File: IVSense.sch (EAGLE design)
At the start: 18 parts

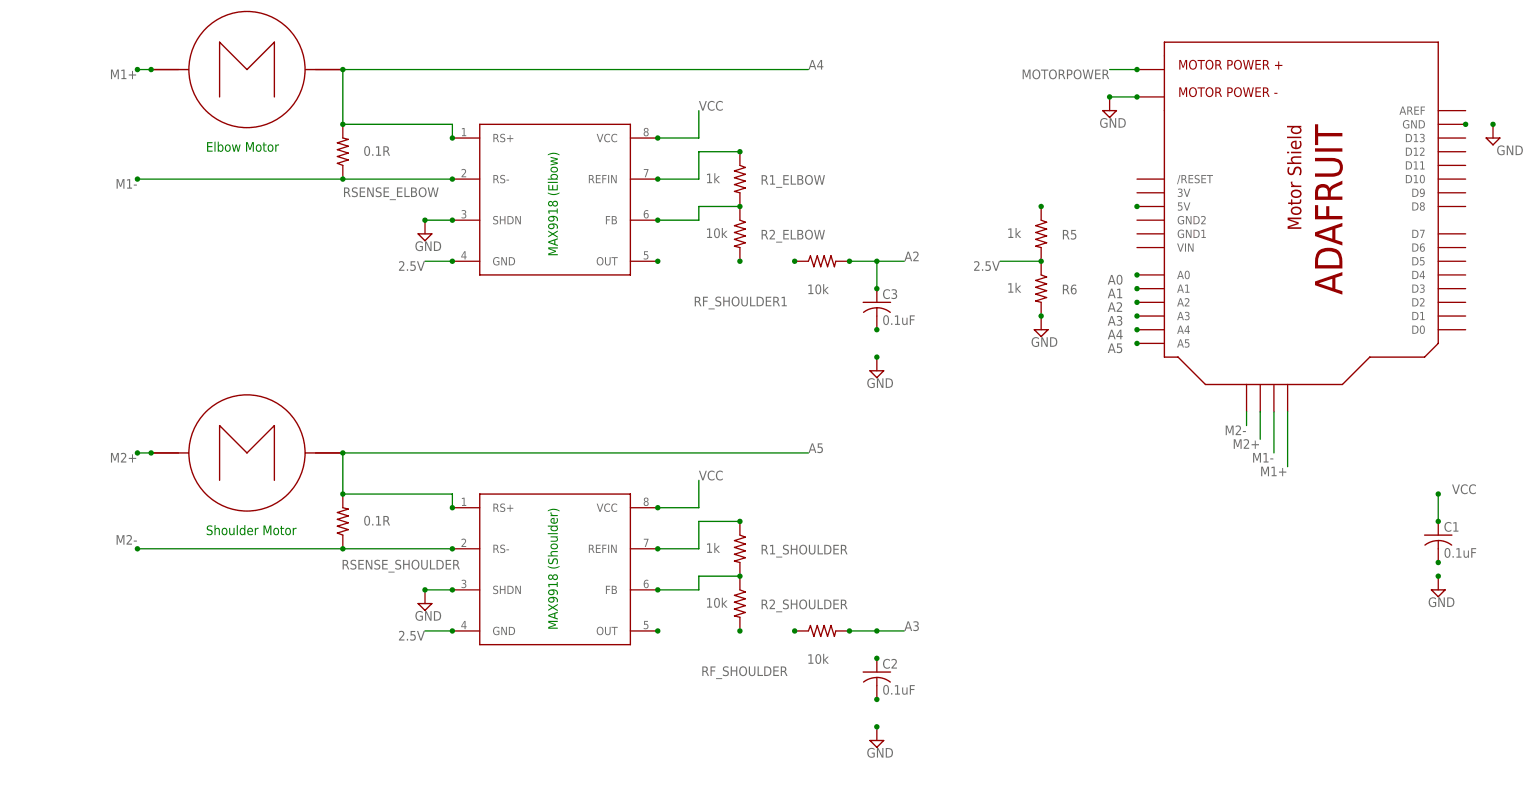
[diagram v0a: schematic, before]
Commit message: update
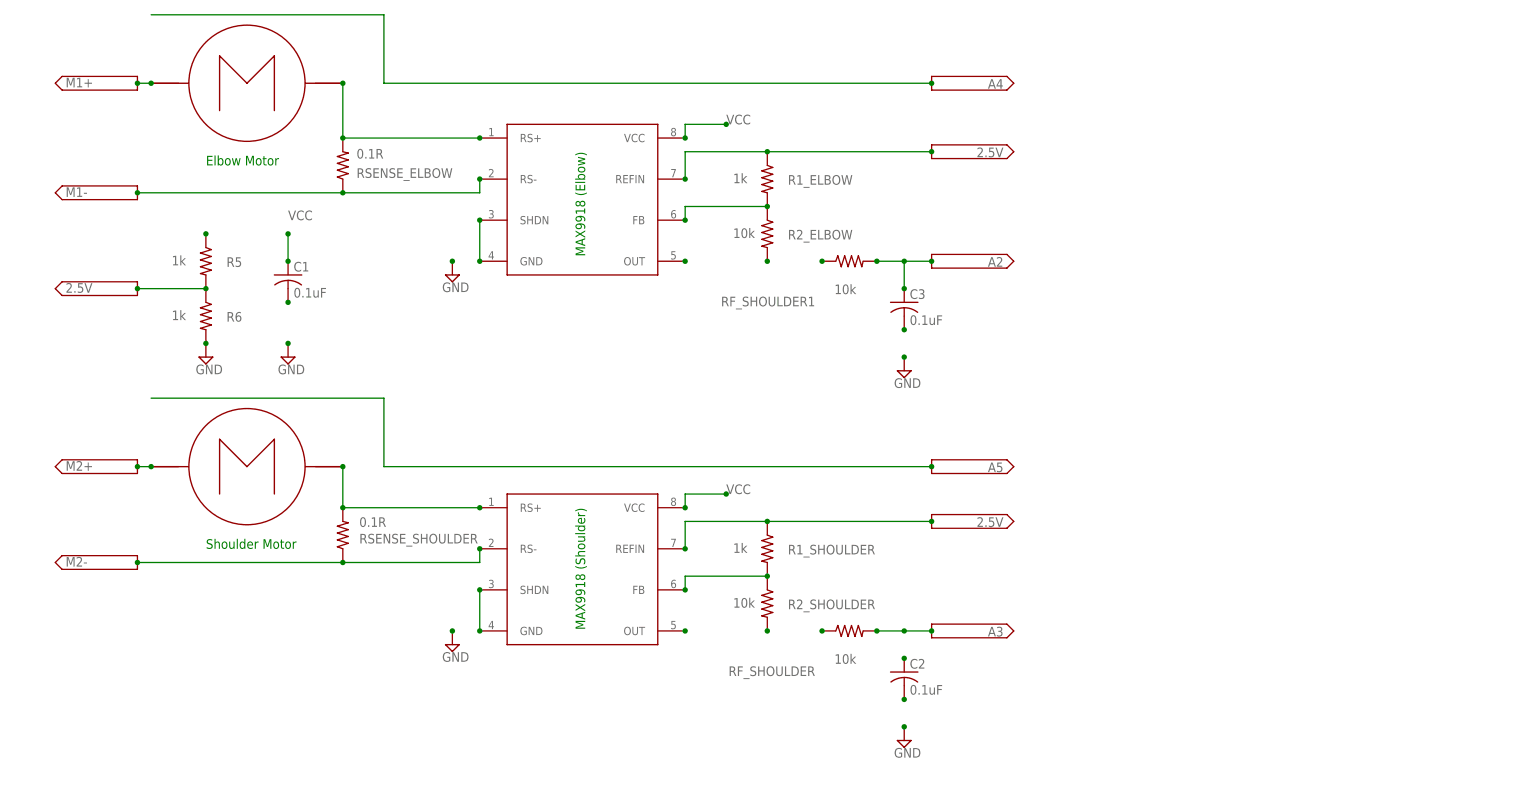
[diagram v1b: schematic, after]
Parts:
- removed U$1: MOTOR_SHIELD, CAP:MOTOR_SHIELD
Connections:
- removed net A0: U$1.A0
- removed net A1: U$1.A1
- removed net A4: MAX9918_ELBOW.RS+, RSENSE_ELBOW.2, U$1.A4, U$4.OUT
- removed net A5: MAX9918_SHOULDER.RS+, RSENSE_SHOULDER.2, U$1.A5, U$5.OUT
- net A2: no longer U$1.A2
- net A3: no longer U$1.A3
- net GND: no longer MAX9918_ELBOW.SHDN, MAX9918_SHOULDER.SHDN
- net N$3: now also MAX9918_ELBOW.RS+, RSENSE_ELBOW.2, U$4.OUT; no longer U$1.5V
- net N$6: now also MAX9918_SHOULDER.RS+, RSENSE_SHOULDER.2, U$5.OUT; no longer U$1.GND
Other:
- note removed: "MOTOR POWER +"
- note removed: "MOTOR POWER -"
- moved on the sheet: C1, C2, C3, R1_ELBOW, R1_SHOULDER, R2_ELBOW, R2_SHOULDER, R5, R6, RF_SHOULDER, RF_SHOULDER1, RSENSE_ELBOW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

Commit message: update
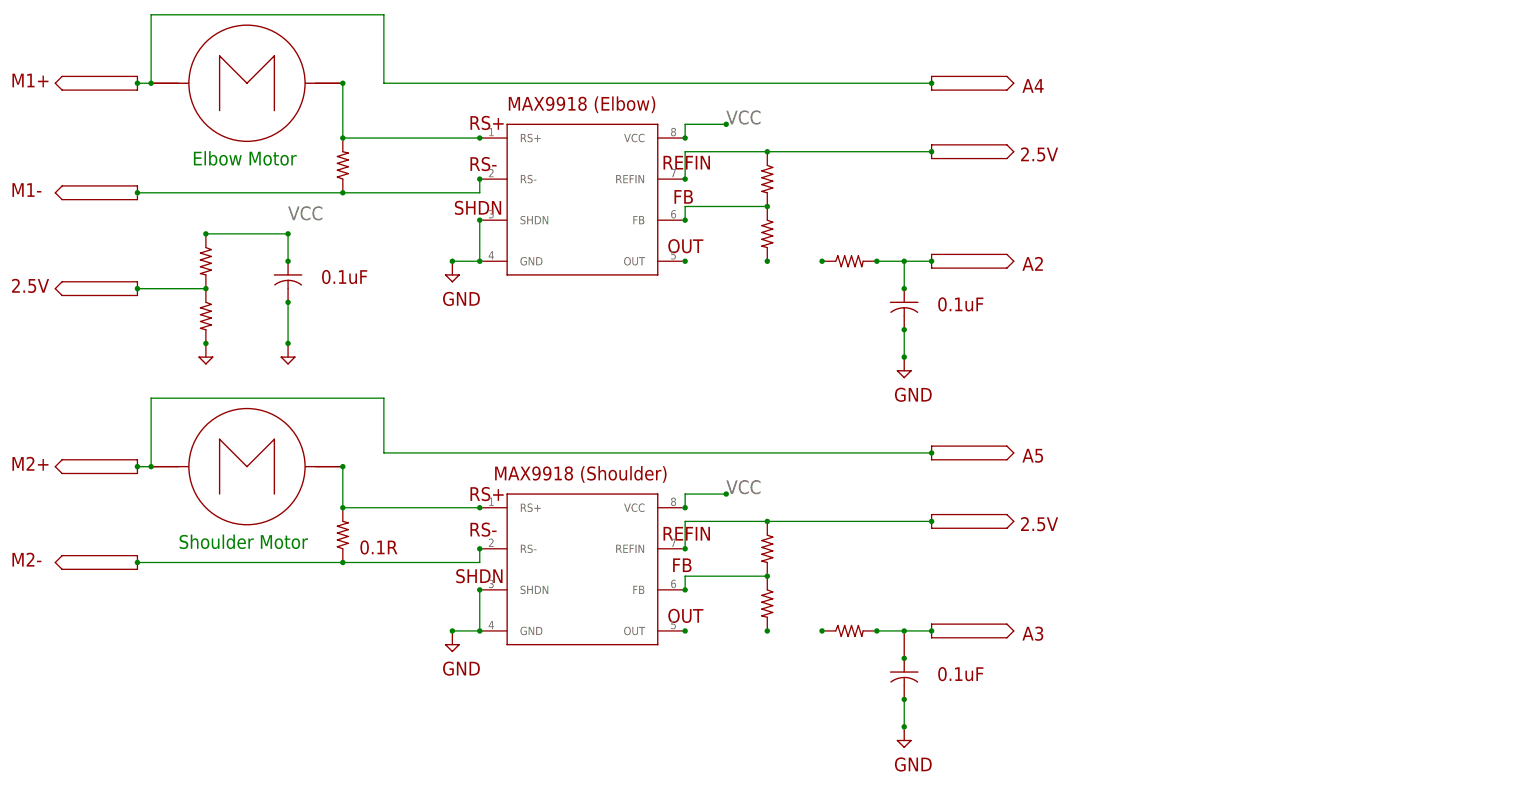
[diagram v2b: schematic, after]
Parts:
- RF_E, RF_S: value 10k -> 4.7k
- renumbered R1_ELBOW to RA_E, R1_SHOULDER to RA_S, R2_ELBOW to RB_E, R2_SHOULDER to RB_S, RF_SHOULDER to RF_S, RF_SHOULDER1 to RF_E, RSENSE_ELBOW to RSENSE_E, RSENSE_SHOULDER to RSENSE_S
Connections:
- removed net N$11: C3.2
- removed net N$12: C2.2
- removed net N$4: R5.1
- removed net N$7: C1.2
- net 2.5V: no longer MAX9918_ELBOW.GND, MAX9918_SHOULDER.GND
- net GND: now also C1.2, C2.2, C3.2, MAX9918_ELBOW.GND, MAX9918_SHOULDER.GND
- net VCC: now also R5.1
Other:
- note added: "FB"
- note added: "OUT"
- note added: "REFIN"
- note added: "RS+"
- note added: "RS-"
- note added: "SHDN"
